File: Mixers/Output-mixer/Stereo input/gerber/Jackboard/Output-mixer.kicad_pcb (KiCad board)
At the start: 2 copper layers, 135 x 110 mm, 131 parts, among them J1 In, J10 In, J11 In, J12 In, J14 Conn_01x04_Female, J17 Conn_01x02_Female, J2 In, J21 Jack 3.5 Out, J22 OutL, J23 OutR, J25 Conn_01x02_Female, J3 In, J4 In, J5 In, J6 In, J7 In, J8 In, J9 In, Q10 2N3904, Q5 2N3904, Q6 2N3904, Q7 2N3904, Q8 2N3904, Q9 2N3904, SW1 Mute, SW2 Mute, SW3 Mute, SW4 Mute, SW5 Mute, SW6 Mute, U1 TL072, U2 TL072, U3 TL072

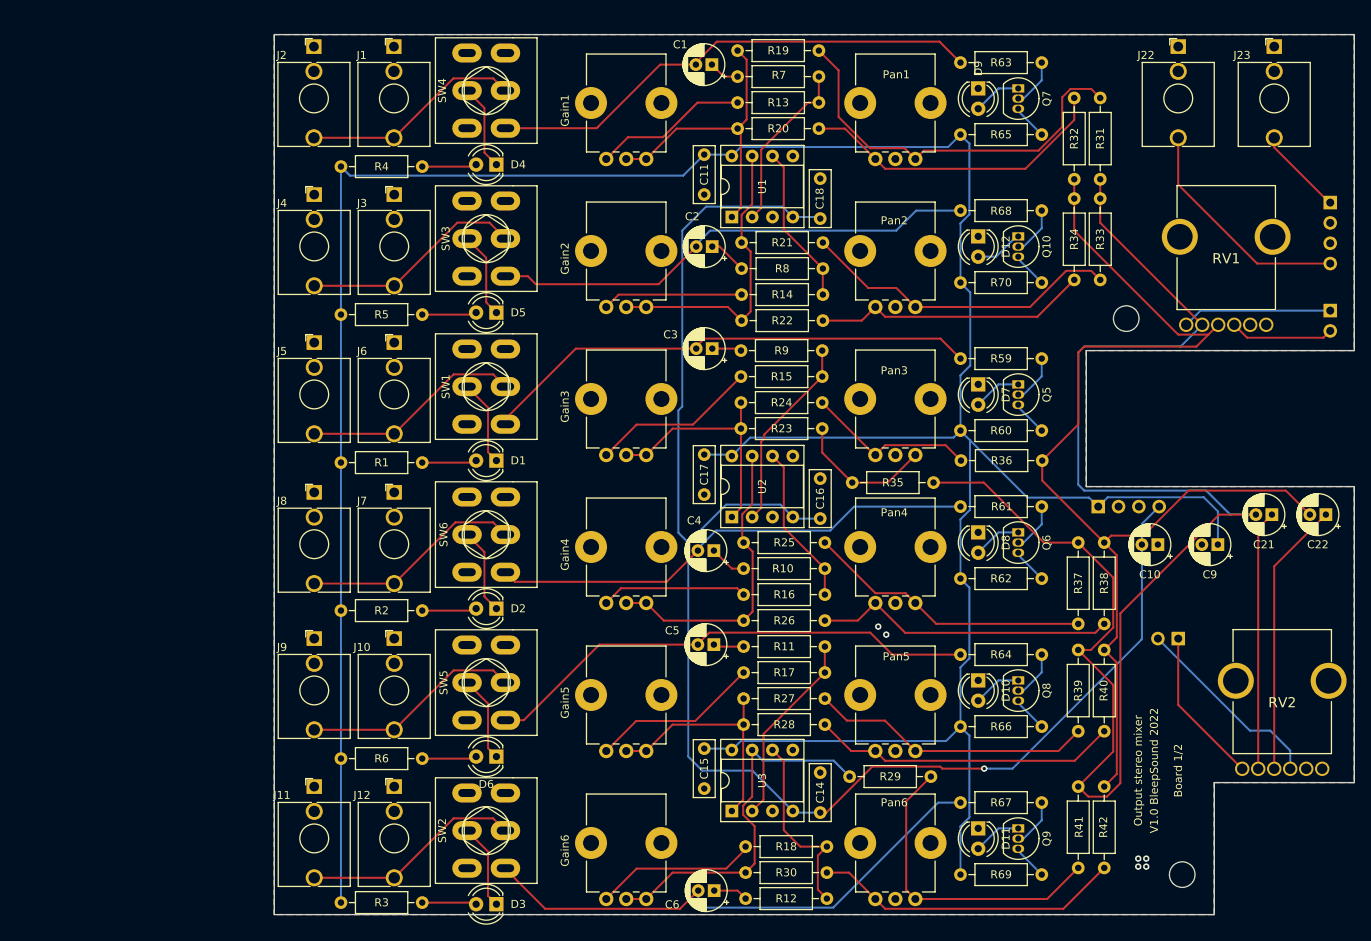
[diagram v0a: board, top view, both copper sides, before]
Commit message: update gerbers for stereo mixer
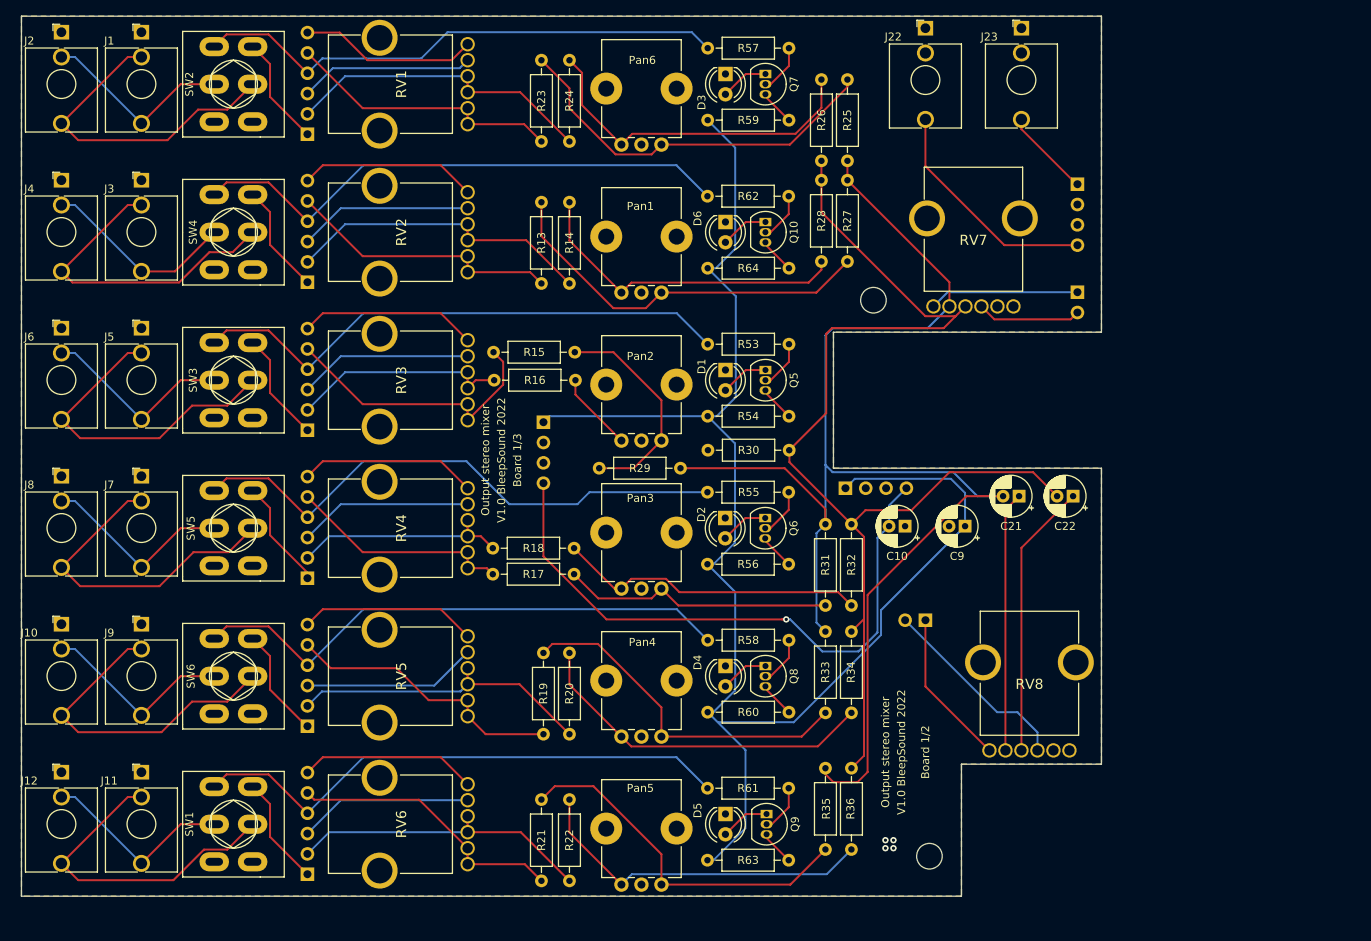
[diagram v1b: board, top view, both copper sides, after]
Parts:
- removed C1, C2, C3, C4, C5, C6: .1µF, Capacitor_THT:CP_Radial_D5.0mm_P2.00mm
- removed C11, C14, C15, C16, C17, C18: 100nF, Capacitor_THT:C_Disc_D7.0mm_W2.5mm_P5.00mm
- removed the D1 at (76.4, 86.5)
- removed the D2 at (76.4, 105.0)
- removed the D3 at (76.4, 142.0)
- removed the D4 at (76.4, 49.5)
- removed the D5 at (76.4, 68.0)
- removed the D6 at (76.4, 123.5)
- removed Gain1, Gain2, Gain3, Gain4, Gain5, Gain6: 500k, Synth:Pot-bourns-alpha
- removed R1, R2, R3, R4, R5, R6: 2.2k, Resistor_THT:R_Axial_DIN0207_L6.3mm_D2.5mm_P10.16mm_Horizontal
- removed R10, R11, R12, R7, R8, R9: 100k, Resistor_THT:R_Axial_DIN0207_L6.3mm_D2.5mm_P10.16mm_Horizontal
- removed the R13 at (106.5, 41.8)
- removed the R14 at (107.0, 65.8)
- removed the R15 at (106.9, 76.0)
- removed the R16 at (107.3, 103.3)
- removed the R17 at (107.3, 113.0)
- removed the R18 at (107.5, 134.8)
- removed U1, U2, U3: TL072, Package_DIP:DIP-8_W7.62mm_Socket
- added J27: Conn_01x06_Female, Connector_PinSocket_2.54mm:PinSocket_1x06_P2.54mm_Vertical, B.Cu at (52.8, 45.8)
- added J28: Conn_01x06_Female, Connector_PinSocket_2.54mm:PinSocket_1x06_P2.54mm_Vertical, B.Cu at (52.8, 64.2)
- added J29: Conn_01x06_Female, Connector_PinSocket_2.54mm:PinSocket_1x06_P2.54mm_Vertical, B.Cu at (52.8, 82.8)
- added J30: Conn_01x06_Female, Connector_PinSocket_2.54mm:PinSocket_1x06_P2.54mm_Vertical, B.Cu at (52.8, 101.2)
- added J35: Conn_01x06_Female, Connector_PinSocket_2.54mm:PinSocket_1x06_P2.54mm_Vertical, B.Cu at (52.8, 119.8)
- added J36: Conn_01x06_Female, Connector_PinSocket_2.54mm:PinSocket_1x06_P2.54mm_Vertical, B.Cu at (52.8, 138.2)
- added J40: Conn_01x04_Female, Connector_PinSocket_2.54mm:PinSocket_1x04_P2.54mm_Vertical, B.Cu at (82.2, 81.8)
- added RV1: 50k, Synth:PTV1124420AA503, F.Cu at (72.8, 42.5)
- added RV2: 50k, Synth:PTV1124420AA503, F.Cu at (72.8, 61.0)
- added RV3: 50k, Synth:PTV1124420AA503, F.Cu at (72.8, 79.5)
- added RV4: 50k, Synth:PTV1124420AA503, F.Cu at (72.8, 98.0)
- added RV5: 50k, Synth:PTV1124420AA503, F.Cu at (72.8, 116.5)
- added RV6: 50k, Synth:PTV1124420AA503, F.Cu at (72.8, 135.0)
- moved J10 41.6 mm to (22.0, 107.0)
- moved J12 41.6 mm to (22.0, 125.5)
- moved J6 41.6 mm to (22.0, 70.0)
- moved R21 40.7 mm to (82.0, 139.1), turned to 90 degrees
- moved R14 35.0 mm to (85.5, 54.2), turned to -90 degrees
- moved R22 33.5 mm to (85.5, 128.9), turned to -90 degrees
- moved R20 33.2 mm to (85.5, 110.6), turned to -90 degrees
- moved R18 32.6 mm to (86.1, 97.5)
- moved R15 32.4 mm to (76.0, 73.0)
- moved R24 32.3 mm to (85.5, 36.5), turned to -90 degrees
- moved Pan1 31.8 mm to (97.0, 65.5)
- moved Pan2 31.8 mm to (97.0, 84.0)
- moved Pan3 31.8 mm to (97.0, 102.5)
- moved Pan4 31.8 mm to (97.0, 121.0)
- moved Pan5 31.8 mm to (97.0, 139.6)
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- renumbered D7 to D1, D8 to D2, D9 to D3, D10 to D4, D11 to D5, D12 to D6, Pan2 to Pan1, Pan3 to Pan2, Pan4 to Pan3, Pan5 to Pan4, Pan6 to Pan5, Pan1 to Pan6, R21 to R13, R22 to R14, R23 to R15, R24 to R16, R25 to R17, R26 to R18, R27 to R19, R28 to R20, R29 to R21, R30 to R22, R19 to R23, R20 to R24, R31 to R25, R32 to R26, R33 to R27, R34 to R28, R35 to R29, R36 to R30, R37 to R31, R38 to R32, R39 to R33, R40 to R34, R41 to R35, R42 to R36, R59 to R53, R60 to R54, R61 to R55, R62 to R56, R63 to R57, R64 to R58, R65 to R59, R66 to R60, R67 to R61, R68 to R62, R69 to R63, R70 to R64, RV1 to RV7, RV2 to RV8, SW2 to SW1, SW4 to SW2, SW1 to SW3, SW3 to SW4, SW6 to SW5, SW5 to SW6
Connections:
- J1 pad TN: unconnected-(J1-PadTN) -> Net-(J1-PadTN)
- J10 pad TN: unconnected-(J10-PadTN) -> Net-(J10-PadTN)
- J11 pad TN: unconnected-(J11-PadTN) -> Net-(J11-PadTN)
- J12 pad T: Net-(J11-PadT) -> Net-(J11-PadTN)
- J12 pad TN: unconnected-(J12-PadTN) -> Net-(J11-PadT)
- J2 pad T: Net-(J1-PadT) -> Net-(J1-PadTN)
- J2 pad TN: unconnected-(J2-PadTN) -> Net-(J1-PadT)
- J3 pad TN: unconnected-(J3-PadTN) -> Net-(J3-PadTN)
- J4 pad T: Net-(J3-PadT) -> Net-(J3-PadTN)
- J4 pad TN: unconnected-(J4-PadTN) -> Net-(J3-PadT)
- J5 pad TN: unconnected-(J5-PadTN) -> Net-(J5-PadTN)
- J6 pad T: Net-(J5-PadT) -> Net-(J5-PadTN)
- J6 pad TN: unconnected-(J6-PadTN) -> Net-(J5-PadT)
- J7 pad TN: unconnected-(J7-PadTN) -> Net-(J7-PadTN)
- J8 pad T: Net-(J7-PadT) -> Net-(J7-PadTN)
- J8 pad TN: unconnected-(J8-PadTN) -> Net-(J7-PadT)
- J9 pad T: Net-(J10-PadT) -> Net-(J10-PadTN)
- J9 pad TN: unconnected-(J9-PadTN) -> Net-(J10-PadT)
- R13 pad 1: Net-(Gain2-Pad1) -> Right2_Out
- R14 pad 2: Net-(Gain2-Pad1) -> Left2_Out
- R15 pad 1: Net-(Gain3-Pad1) -> Right3_Out
- R16 pad 2: Net-(Gain3-Pad1) -> Left3_Out
- R17 pad 1: Net-(Gain4-Pad1) -> Right4_Out
- R18 pad 2: Net-(Gain4-Pad1) -> Left4_Out
- R19 pad 1: Net-(Gain5-Pad1) -> Right5_Out
- R20 pad 2: Net-(Gain5-Pad1) -> Left5_Out
- R21 pad 1: Net-(Gain6-Pad1) -> Right6_Out
- R22 pad 2: Net-(Gain6-Pad1) -> Left6_Out
- R23 pad 1: Net-(Gain1-Pad1) -> Right1_Out
- R24 pad 2: Net-(Gain1-Pad1) -> Left1_Out
- R53 pad 1: In3 -> Right3_In
- R55 pad 1: In4 -> Right4_In
- R57 pad 1: In1 -> Right1_In
- R58 pad 1: In5 -> Right5_In
- R61 pad 1: In6 -> Right6_In
- R62 pad 1: In2 -> Right2_In
- SW1 pad 1: GND -> Right6_In
- SW1 pad 2: Net-(D3-Pad1) -> Net-(J11-PadT)
- SW1 pad 4: unconnected-(SW2-Pad4) -> Left6_In
- SW1 pad 5: Net-(J11-PadT) -> Net-(J11-PadTN)
- SW1 pad 6: In6 -> unconnected-(SW1-Pad6)
- SW2 pad 1: GND -> Right1_In
- SW2 pad 2: Net-(D4-Pad1) -> Net-(J1-PadT)
- SW2 pad 4: unconnected-(SW4-Pad4) -> Left1_In
- SW2 pad 5: Net-(J1-PadT) -> Net-(J1-PadTN)
- SW2 pad 6: In1 -> unconnected-(SW2-Pad6)
- SW3 pad 1: GND -> Right3_In
- SW3 pad 2: Net-(D1-Pad1) -> Net-(J5-PadT)
- SW3 pad 4: unconnected-(SW1-Pad4) -> Left3_In
- SW3 pad 5: Net-(J5-PadT) -> Net-(J5-PadTN)
- SW3 pad 6: In3 -> unconnected-(SW3-Pad6)
- SW4 pad 1: GND -> Right2_In
- SW4 pad 2: Net-(D5-Pad1) -> Net-(J3-PadT)
- SW4 pad 4: unconnected-(SW3-Pad4) -> Left2_In
- SW4 pad 5: Net-(J3-PadT) -> Net-(J3-PadTN)
- SW4 pad 6: In2 -> unconnected-(SW4-Pad6)
- SW5 pad 1: GND -> Right4_In
- SW5 pad 2: Net-(D2-Pad1) -> Net-(J7-PadT)
- SW5 pad 4: unconnected-(SW6-Pad4) -> Left4_In
- SW5 pad 5: Net-(J7-PadT) -> Net-(J7-PadTN)
- SW5 pad 6: In4 -> unconnected-(SW5-Pad6)
- SW6 pad 1: GND -> Right5_In
- SW6 pad 2: Net-(D6-Pad1) -> Net-(J10-PadTN)
- SW6 pad 4: unconnected-(SW5-Pad4) -> Left5_In
- SW6 pad 6: In5 -> unconnected-(SW6-Pad6)
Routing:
- net +12V: track 376.0 -> 194.5 mm
- net -12V: track 191.0 -> 76.3 mm
- net Right4_In: track 0.00 -> 70.0 mm
- net Right5_In: track 0.00 -> 68.8 mm
- net Right3_In: track 0.00 -> 68.8 mm
- net Right2_In: track 0.00 -> 68.8 mm
- net Right6_In: track 0.00 -> 68.8 mm
- net Right1_In: track 0.00 -> 67.3 mm
- net In6: track 67.0 -> 0.00 mm
- net In3: track 62.9 -> 0.00 mm
- net In5: track 62.6 -> 0.00 mm
- net In1: track 62.6 -> 0.00 mm
- net In4: track 61.4 -> 0.00 mm
- net In2: track 61.3 -> 0.00 mm
- net Net-(Gain6-Pad1): track 46.7 -> 0.00 mm
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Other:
- board text added: "Board 1/3"
